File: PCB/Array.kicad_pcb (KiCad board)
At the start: 2 copper layers, 95.2 x 95.2 mm, 55 parts, among them SW1 SW_Push, SW10 SW_Push, SW2 SW_Push, SW3 SW_Push, SW4 SW_Push, SW5 SW_Push, SW6 SW_Push, SW7 SW_Push, SW8 SW_Push, SW9 SW_Push, U1 AD009-06H, U2 AD009-06H, U3 AD009-06H, U4 AD009-06H, U5 AD009-06H

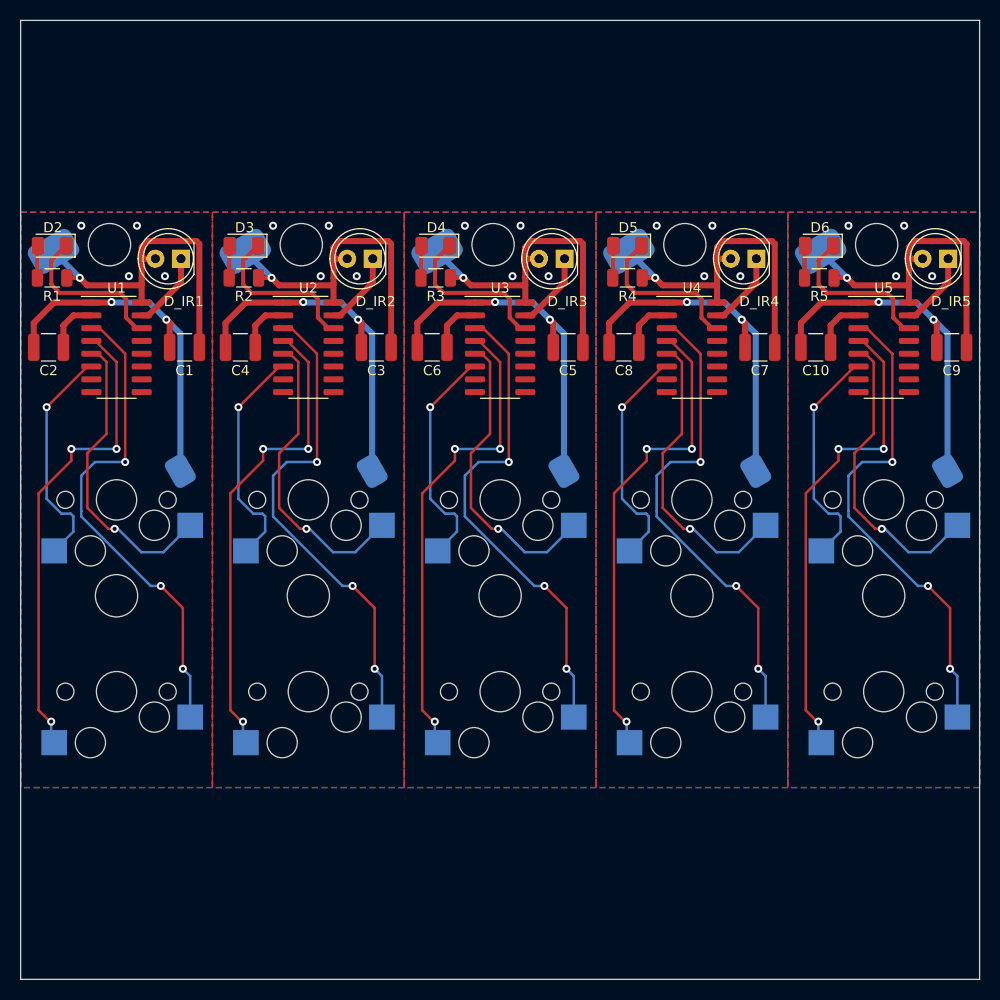
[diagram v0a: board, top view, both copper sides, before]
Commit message: 2nd
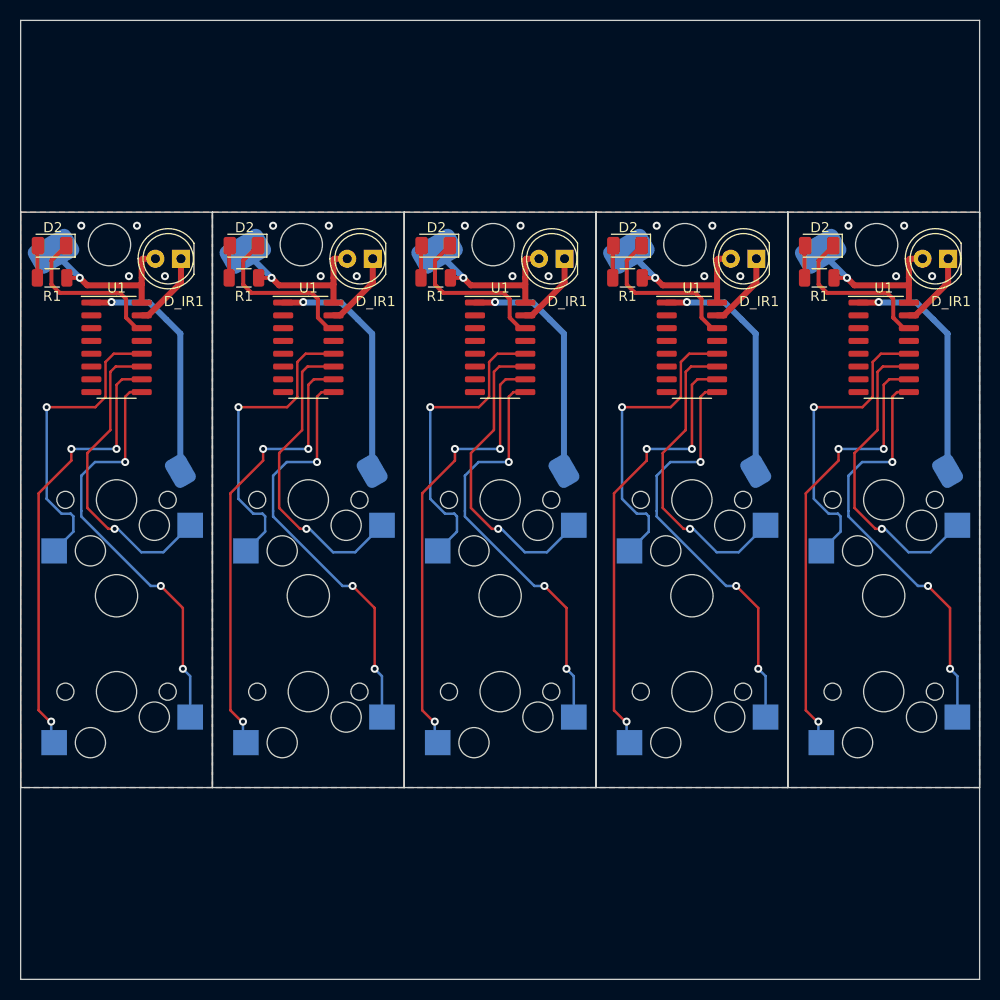
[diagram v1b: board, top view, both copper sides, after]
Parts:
- removed BT2, BT3, BT4, BT5: 3V, ktRMT_Thumb:CR16xx_Holder
- removed C1, C10, C2, C3, C4, C5, C6, C7, C8, C9: 47uF/16V, Capacitor_SMD:C_1210_3225Metric
- removed D3, D4, D5, D6: LED, LED_SMD:LED_1206_3216Metric
- removed D_IR2, D_IR3, D_IR4, D_IR5: LED, LED_THT:LED_D5.0mm
- removed R2, R3, R4, R5: 470oum, Resistor_SMD:R_1206_3216Metric
- removed REF**1, REF**2, REF**3, REF**4, REF**5, REF**6, REF**7, REF**8: Hole_4P2, ktRMT_Thumb:Hole_4P2
- removed SW10, SW3, SW4, SW5, SW6, SW7, SW8, SW9: SW_Push, ktRMT_Thumb:MX_Socket
- removed U2, U3, U4, U5: AD009-06H, Package_SO:SOP-16_3.9x9.9mm_P1.27mm
- added BT1: 3V, ktRMT_Thumb:CR16xx_Holder, F.Cu at (28.6, 28.6)
- added BT1: 3V, ktRMT_Thumb:CR16xx_Holder, F.Cu at (85.7, 28.6)
- added BT1: 3V, ktRMT_Thumb:CR16xx_Holder, F.Cu at (66.7, 28.6)
- added BT1: 3V, ktRMT_Thumb:CR16xx_Holder, F.Cu at (47.6, 28.6)
- added D2: LED, LED_SMD:LED_1206_3216Metric, F.Cu at (22.2, 22.4)
- added D2: LED, LED_SMD:LED_1206_3216Metric, F.Cu at (79.3, 22.4)
- added D2: LED, LED_SMD:LED_1206_3216Metric, F.Cu at (60.3, 22.4)
- added D2: LED, LED_SMD:LED_1206_3216Metric, F.Cu at (41.2, 22.4)
- added D_IR1: LED, LED_THT:LED_D5.0mm, F.Cu at (73.1, 23.7)
- added D_IR1: LED, LED_THT:LED_D5.0mm, F.Cu at (35.0, 23.7)
- added D_IR1: LED, LED_THT:LED_D5.0mm, F.Cu at (92.1, 23.7)
- added D_IR1: LED, LED_THT:LED_D5.0mm, F.Cu at (54.0, 23.7)
- added R1: 470oum, Resistor_SMD:R_1206_3216Metric, F.Cu at (41.2, 25.6)
- added R1: 470oum, Resistor_SMD:R_1206_3216Metric, F.Cu at (60.3, 25.6)
- added R1: 470oum, Resistor_SMD:R_1206_3216Metric, F.Cu at (79.3, 25.6)
- added R1: 470oum, Resistor_SMD:R_1206_3216Metric, F.Cu at (22.2, 25.6)
- added REF**: Hole_4P2, ktRMT_Thumb:Hole_4P2, F.Cu at (85.7, 57.1)
- added REF**: Hole_4P2, ktRMT_Thumb:Hole_4P2, F.Cu at (66.0, 22.3)
- added REF**: Hole_4P2, ktRMT_Thumb:Hole_4P2, F.Cu at (27.9, 22.3)
- added REF**: Hole_4P2, ktRMT_Thumb:Hole_4P2, F.Cu at (46.9, 22.3)
- added REF**: Hole_4P2, ktRMT_Thumb:Hole_4P2, F.Cu at (28.6, 57.1)
- added REF**: Hole_4P2, ktRMT_Thumb:Hole_4P2, F.Cu at (66.7, 57.1)
- added REF**: Hole_4P2, ktRMT_Thumb:Hole_4P2, F.Cu at (85.0, 22.3)
- added REF**: Hole_4P2, ktRMT_Thumb:Hole_4P2, F.Cu at (47.6, 57.1)
- added SW1: SW_Push, ktRMT_Thumb:MX_Socket, F.Cu at (28.6, 47.6)
- added SW1: SW_Push, ktRMT_Thumb:MX_Socket, F.Cu at (47.6, 47.6)
- added SW1: SW_Push, ktRMT_Thumb:MX_Socket, F.Cu at (85.7, 47.6)
- added SW1: SW_Push, ktRMT_Thumb:MX_Socket, F.Cu at (66.7, 47.6)
- added SW2: SW_Push, ktRMT_Thumb:MX_Socket, F.Cu at (66.7, 66.7)
- added SW2: SW_Push, ktRMT_Thumb:MX_Socket, F.Cu at (85.7, 66.7)
- added SW2: SW_Push, ktRMT_Thumb:MX_Socket, F.Cu at (47.6, 66.7)
- added SW2: SW_Push, ktRMT_Thumb:MX_Socket, F.Cu at (28.6, 66.7)
- added U1: HB1531E, Package_SO:SOP-16_3.9x9.9mm_P1.27mm, F.Cu at (47.6, 32.5)
- added U1: HB1531E, Package_SO:SOP-16_3.9x9.9mm_P1.27mm, F.Cu at (85.7, 32.5)
- added U1: HB1531E, Package_SO:SOP-16_3.9x9.9mm_P1.27mm, F.Cu at (28.6, 32.5)
- added U1: HB1531E, Package_SO:SOP-16_3.9x9.9mm_P1.27mm, F.Cu at (66.7, 32.5)
- U1: value AD009-06H -> HB1531E
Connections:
- SW1 pad 2: Net-(SW1-Pad2) -> Net-(U1-Pad11)
- SW2 pad 1: Net-(SW2-Pad1) -> Net-(U1-Pad10)
- U1 pad 10: unconnected-(U1-Pad10) -> Net-(U1-Pad10)
- U1 pad 11: unconnected-(U1-Pad11) -> Net-(U1-Pad11)
- U1 pad 12: unconnected-(U1-Pad12) -> Net-(SW1-Pad1)
- U1 pad 2: Net-(C2-Pad2) -> unconnected-(U1-Pad2)
- U1 pad 3: Net-(SW2-Pad2) -> unconnected-(U1-Pad3)
- U1 pad 4: Net-(SW2-Pad1) -> unconnected-(U1-Pad4)
- U1 pad 5: Net-(SW1-Pad2) -> unconnected-(U1-Pad5)
- U1 pad 6: Net-(SW1-Pad1) -> unconnected-(U1-Pad6)
- U1 pad 9: unconnected-(U1-Pad9) -> Net-(SW2-Pad2)
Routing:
- net Net-(SW2-Pad1): track 238.6 -> 0.00 mm, vias 15 -> 0
- net Net-(U1-Pad10): track 0.00 -> 224.1 mm, vias 0 -> 15
- net Net-(U1-Pad11): track 0.00 -> 154.7 mm, vias 0 -> 5
- net Net-(SW1-Pad2): track 151.4 -> 0.00 mm, vias 5 -> 0
- net Net-(BT1-Pad1): track 173.9 -> 85.8 mm
- net Net-(BT1-Pad2): track 178.4 -> 119.1 mm, vias 30 -> 25
- net Net-(SW1-Pad1): track 114.1 -> 151.9 mm
- net Net-(SW2-Pad2): track 245.6 -> 211.4 mm
- net Net-(C2-Pad2): track 26.8 -> 0.00 mm
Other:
- outline, holes or cut-outs redrawn
